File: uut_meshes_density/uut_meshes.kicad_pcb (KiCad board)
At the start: 13 copper layers, 100 x 100 mm, 9 parts, among them J1 Conn_02x10_Counter_Clockwise, J2 Conn_02x10_Counter_Clockwise, J3 Conn_02x10_Counter_Clockwise, J4 Conn_02x10_Counter_Clockwise, J5 MeshAnchor_2W_T0.200mm_S0.200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, J6 MeshAnchor_2W_T0.150mm_S0.150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, J7 MeshAnchor_2W_T0.300mm_S0.300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, J8 MeshAnchor_2W_T0.500mm_S0.500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

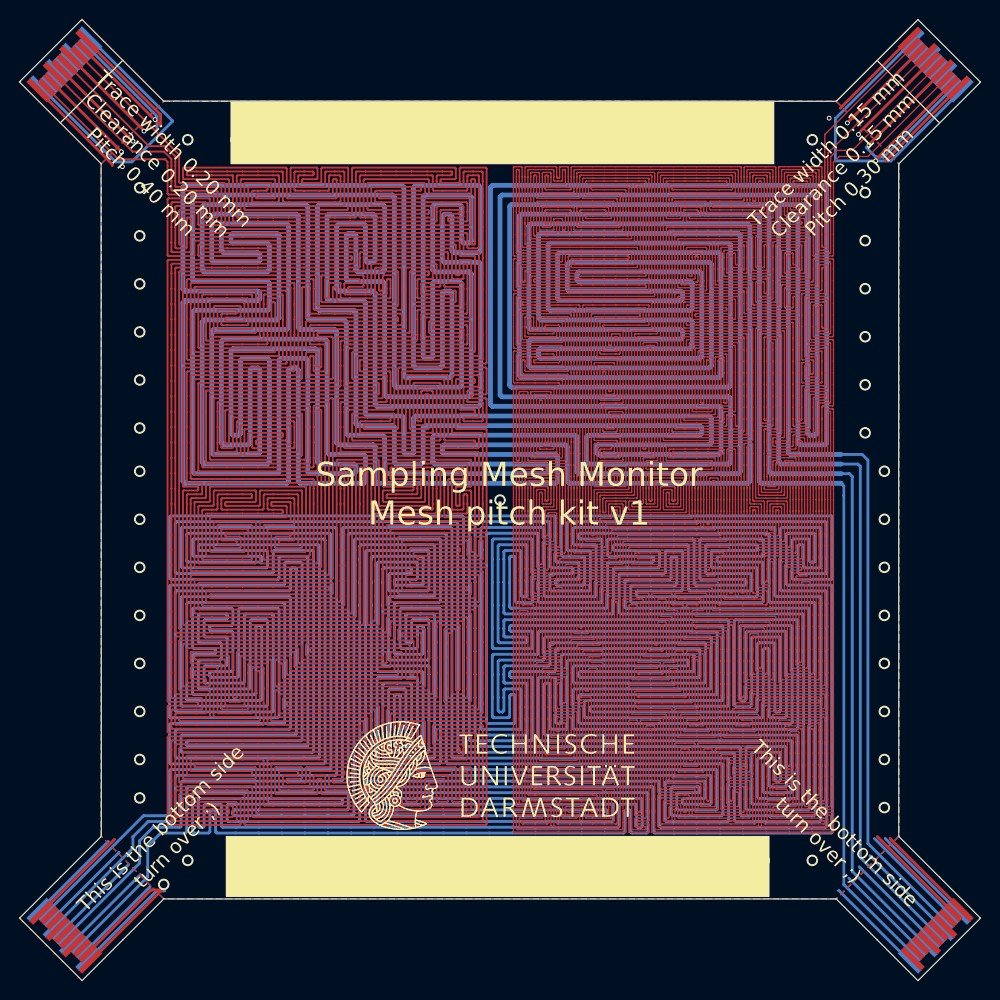
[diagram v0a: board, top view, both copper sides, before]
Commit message: Add new mesh coupons
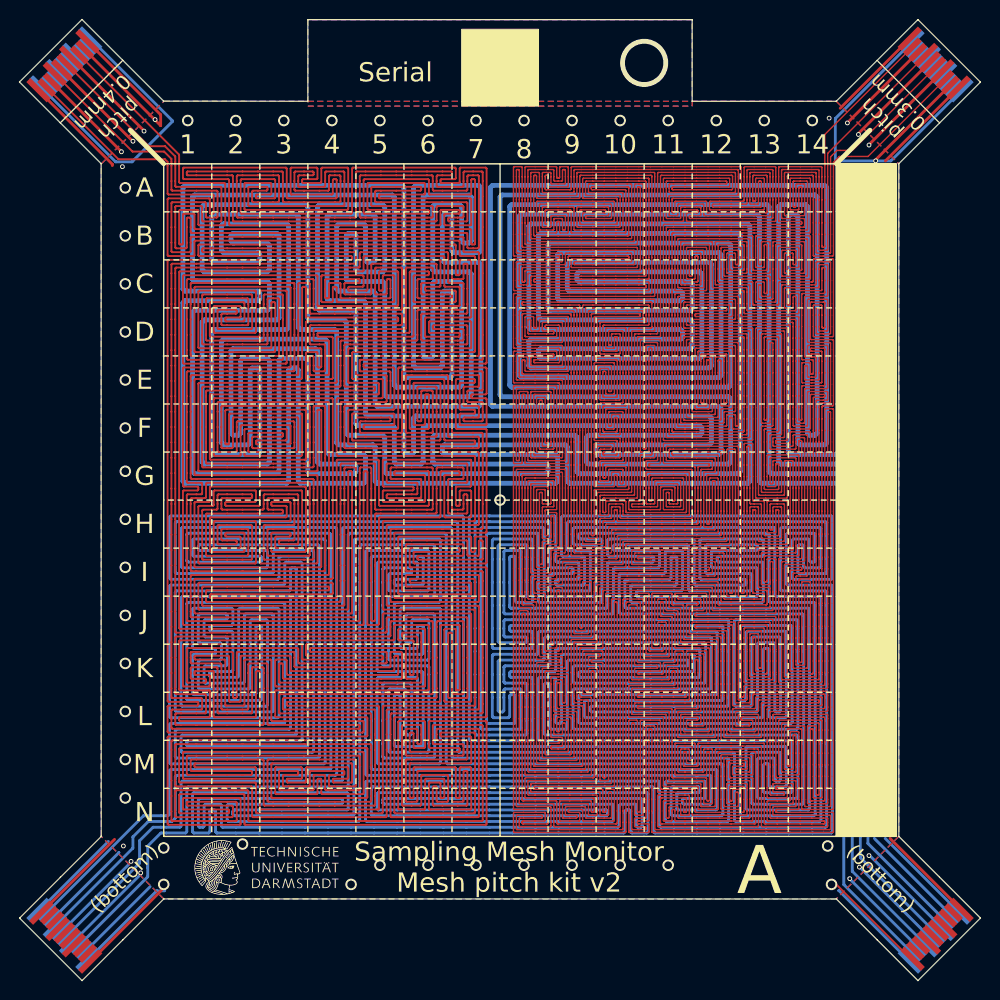
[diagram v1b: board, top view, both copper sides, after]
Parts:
- removed logo_tu_darmstadt_30.0mm: G*****, logo_tu_darmstadt:logo_tu_darmstadt_30.0mm
- added logo_tu_darmstadt_15.0mm: G*****, logo_tu_darmstadt:logo_tu_darmstadt_15.0mm, F.Cu at (118.2, 135.4)
- added logo_tu_darmstadt_15.0mm: G*****, logo_tu_darmstadt:logo_tu_darmstadt_15.0mm, B.Cu at (183.5, 135.4)
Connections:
- J1 pad 9: GND -> unconnected-(J1-Pin_9-Pad9)
- J3 pad 13: unconnected-(J3-Pin_13-Pad13) -> Net-(J3-Pin_13)
- J3 pad 15: unconnected-(J3-Pin_15-Pad15) -> Net-(J3-Pin_15)
- J3 pad 17: unconnected-(J3-Pin_17-Pad17) -> Net-(J3-Pin_17)
- J3 pad 19: unconnected-(J3-Pin_19-Pad19) -> Net-(J3-Pin_19)
- J3 pad 9: GND -> unconnected-(J3-Pin_9-Pad9)
- J4 pad 9: GND -> unconnected-(J4-Pin_9-Pad9)
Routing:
- net (no net): track 0.00 -> 19452.7 mm
- net mesh0: track 13591.9 -> 0.00 mm
- net mesh1: track 5860.9 -> 0.00 mm
- net GND: track 393.3 -> 358.7 mm, vias 68 -> 73
- net unconnected-(J3-Pin_17-Pad17): track 16.2 -> 0.00 mm
- net Net-(J3-Pin_17): track 0.00 -> 16.2 mm
- net unconnected-(J3-Pin_19-Pad19): track 16.1 -> 0.00 mm
- net Net-(J3-Pin_19): track 0.00 -> 16.1 mm
- net unconnected-(J3-Pin_15-Pad15): track 15.8 -> 0.00 mm
- net Net-(J3-Pin_15): track 0.00 -> 15.8 mm
- net unconnected-(J3-Pin_13-Pad13): track 15.2 -> 0.00 mm
- net Net-(J3-Pin_13): track 0.00 -> 15.2 mm
- removed copper zone on User.1, net GND
- removed copper zone on User.2, net GND
- removed copper zone on User.3, net GND
- removed copper zone on User.4, net GND
- removed copper zone on User.5, net GND
- removed copper zone on User.6, net GND
- removed copper zone on User.7, net GND
- removed copper zone on User.8, net GND
- removed copper zone on User.9, net GND
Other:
- outline, holes or cut-outs redrawn
- copper layers 13 -> 4
- board text added: "(bottom)"
- board text added: "1"
- board text added: "10"
- board text added: "11"
- board text added: "12"
- board text added: "13"
- board text added: "14"
- board text added: "2"
- board text added: "3"
- board text added: "4"
- board text added: "5"
- board text added: "6"
- board text added: "7"
- board text added: "8"
- board text added: "9"
- board text added: "A"
- board text added: "B"
- board text added: "C"
- board text added: "D"
- board text added: "E"
- board text added: "F"
- board text added: "G"
- board text added: "H"
- board text added: "I"
- board text added: "J"
- board text added: "K"
- board text added: "L"
- board text added: "M"
- board text added: "N"
- board text added: "Sampling Mesh Monitor Mesh pitch kit v2"
- board text added: "Serial"
- board text added: "pitch 0.3mm"
- board text added: "pitch 0.4mm"
- board text added: "pitch 0.60mm"
- board text added: "pitch 1.00mm"
- board text removed: "Sampling Mesh Monitor Mesh pitch kit v1"
- board text removed: "This is the bottom side turn over ;)"
- board text removed: "Trace width 0.15 mm Clearance 0.15 mm Pitch 0.30 mm"
- board text removed: "Trace width 0.20 mm Clearance 0.20 mm Pitch 0.40 mm"
- board text removed: "Trace width 0.30 mm Clearance 0.30 mm Pitch 0.60 mm"
- board text removed: "Trace width 0.50 mm Clearance 0.50 mm Pitch 1.00 mm"
